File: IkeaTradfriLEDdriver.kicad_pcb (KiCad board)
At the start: 2 copper layers, 89.5 x 44.4 mm, 16 parts, among them J1 input, J2 IKEA Zigbit module, J3 led strip, Q1 BUZ11, Q2 BC547, U1 LM741, U2 LM1117-3.3

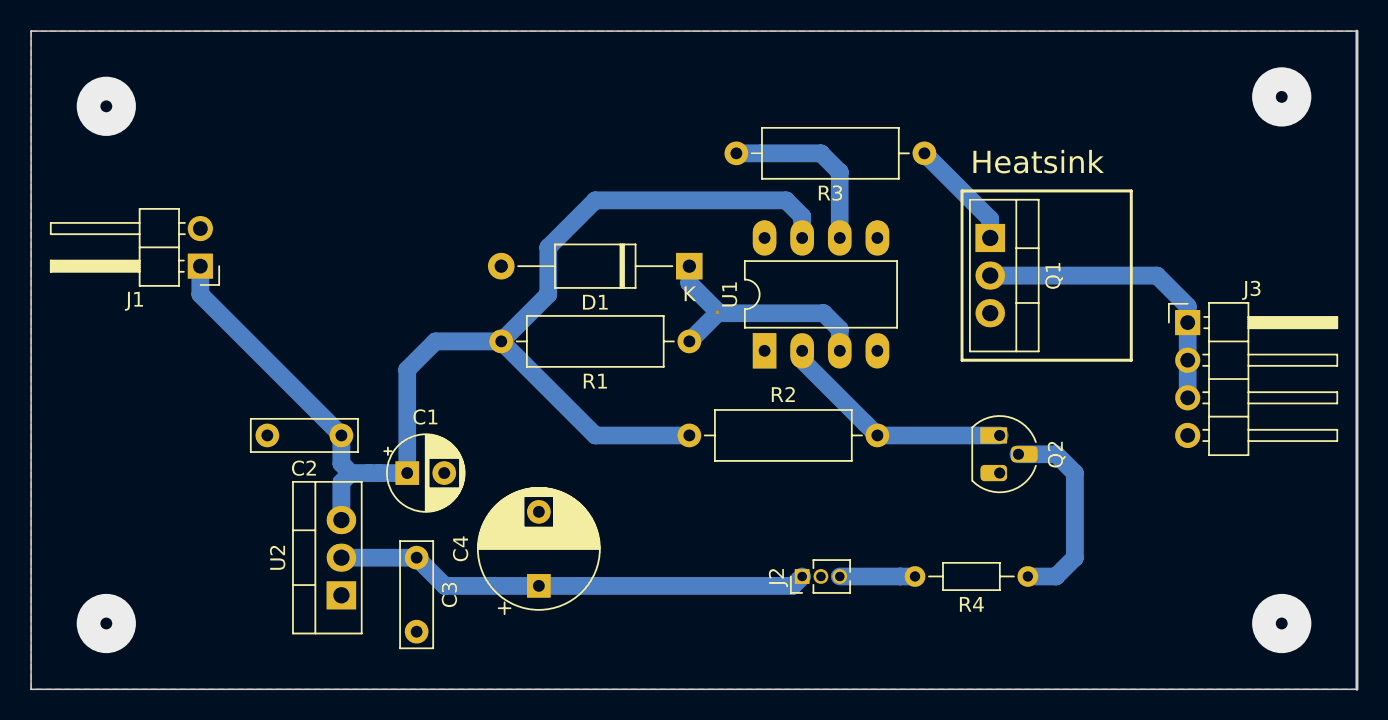
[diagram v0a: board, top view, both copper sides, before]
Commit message: Provedene opravy na desce
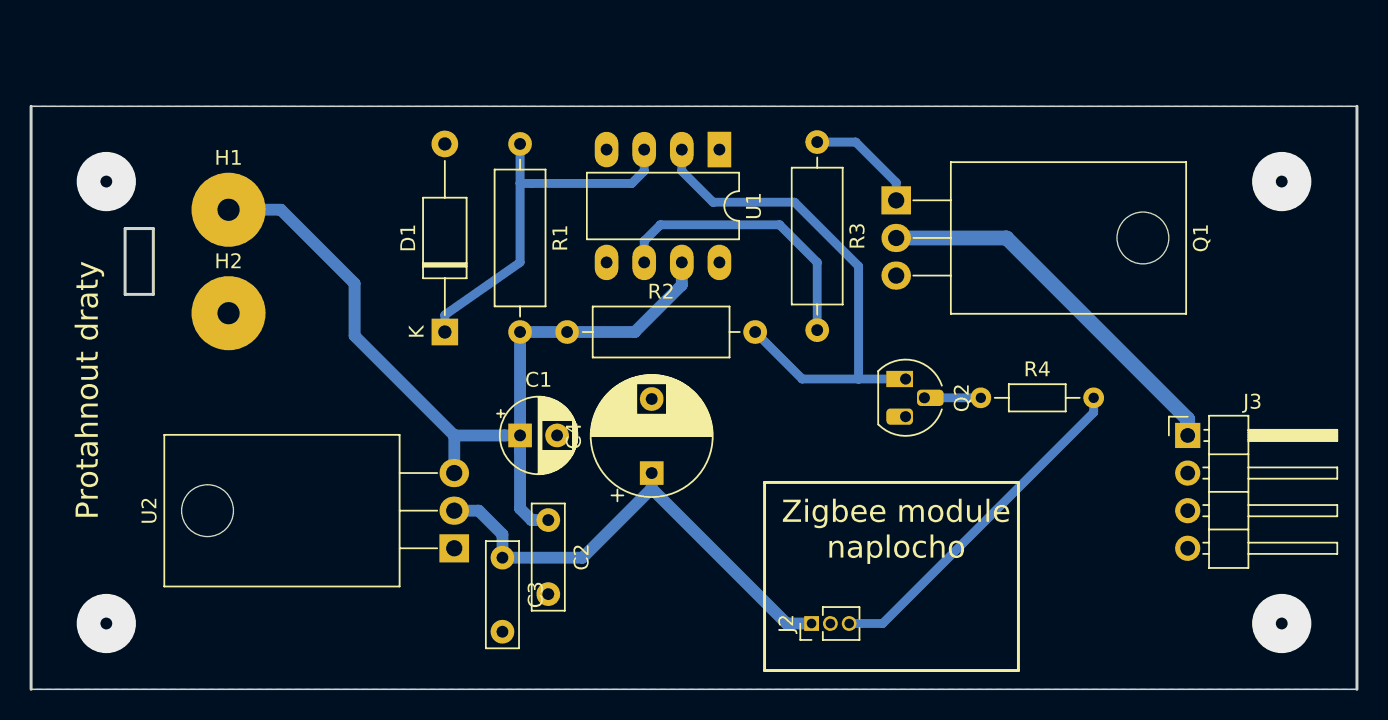
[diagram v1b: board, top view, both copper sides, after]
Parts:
- removed J1: input, Connector_PinHeader_2.54mm:PinHeader_1x02_P2.54mm_Horizontal
- added H1: +, MountingHole:MountingHole_2.5mm_Pad, F.Cu at (108.6, 76.2)
- added H2: -, MountingHole:MountingHole_2.5mm_Pad, F.Cu at (108.6, 83.2)
- Q1, U2: footprint Package_TO_SOT_THT:TO-220-3_Vertical -> Package_TO_SOT_THT:TO-220-3_Horizontal_TabDown
- moved R1 17.6 mm to (128.3, 71.8), turned to 270 degrees
- moved D1 17.1 mm to (123.2, 84.5), turned to 90 degrees
- moved C2 15.1 mm to (130.2, 97.2), turned to 270 degrees
- moved U1 13.9 mm to (141.7, 72.1), turned to 270 degrees
- moved R4 12.5 mm to (159.4, 88.9), turned to 0 degrees
- moved R2 10.8 mm to (131.4, 84.5)
- moved C4 10.8 mm to (137.2, 94.0)
- moved U2 8.26 mm to (123.8, 99.1)
- moved C1 8.03 mm to (128.3, 91.4)
- moved J3 7.62 mm to (173.4, 91.4)
- moved Q2 7.41 mm to (154.3, 87.6)
- moved R3 7.28 mm to (148.3, 71.6), turned to 270 degrees
- moved Q1 6.84 mm to (153.7, 75.6)
- moved C3 5.80 mm to (127.1, 99.7)
- moved J2 3.24 mm to (148.0, 104.1)
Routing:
- net +12V: track 84.2 -> 58.5 mm
- net Net-(Q2-Pad1): track 16.1 -> 35.1 mm
- net pwm: track 5.08 -> 23.4 mm
- net Net-(Q2-Pad2): track 13.8 -> 3.81 mm
- net Net-(D1-Pad1): track 16.8 -> 25.5 mm
- net Net-(R3-Pad2): track 12.4 -> 19.2 mm
- net Net-(J3-Pad1): track 20.4 -> 25.9 mm
- net +3V3: track 32.2 -> 33.1 mm
- removed copper zone on F.Cu, net GND
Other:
- board size 89.5 x 44.4 mm -> 89.5 x 39.4 mm
- board text added: "Protahnout draty"
- board text added: "Zigbee module naplocho"
- board text removed: "Heatsink"
